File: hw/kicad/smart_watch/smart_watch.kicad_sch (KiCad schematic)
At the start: 11 parts, among them U1 STM32L476RG, U2 GC9A01, U3 LIS2MDL, U4 SHT41

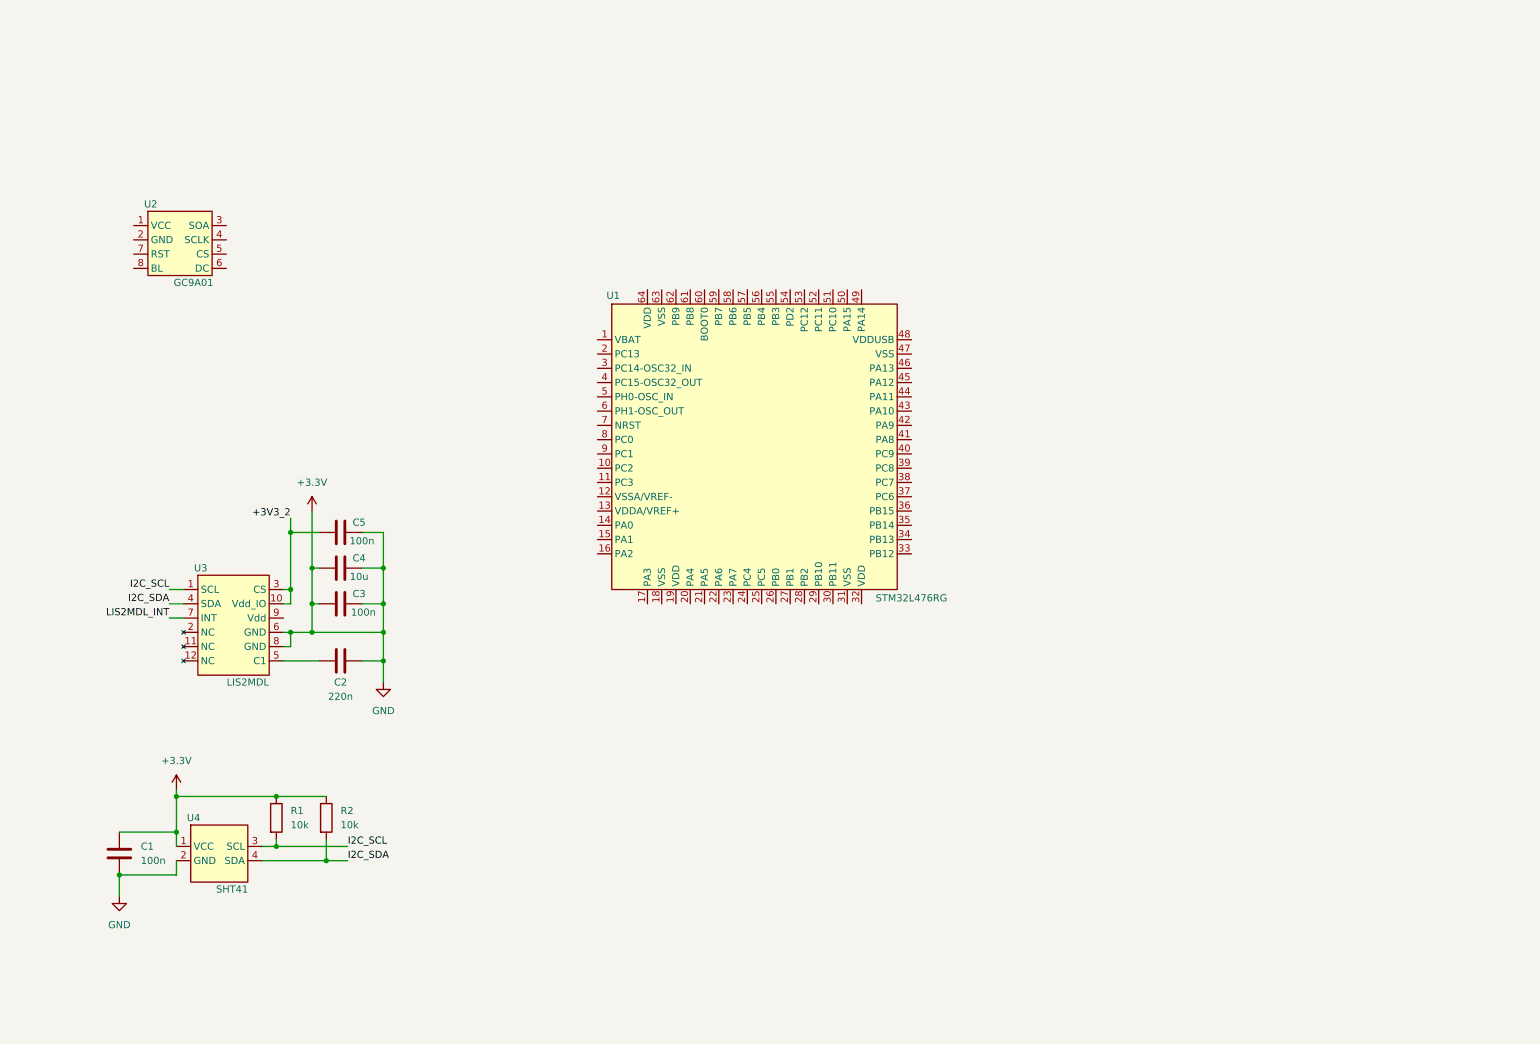
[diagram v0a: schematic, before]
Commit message: work on kicad schematic
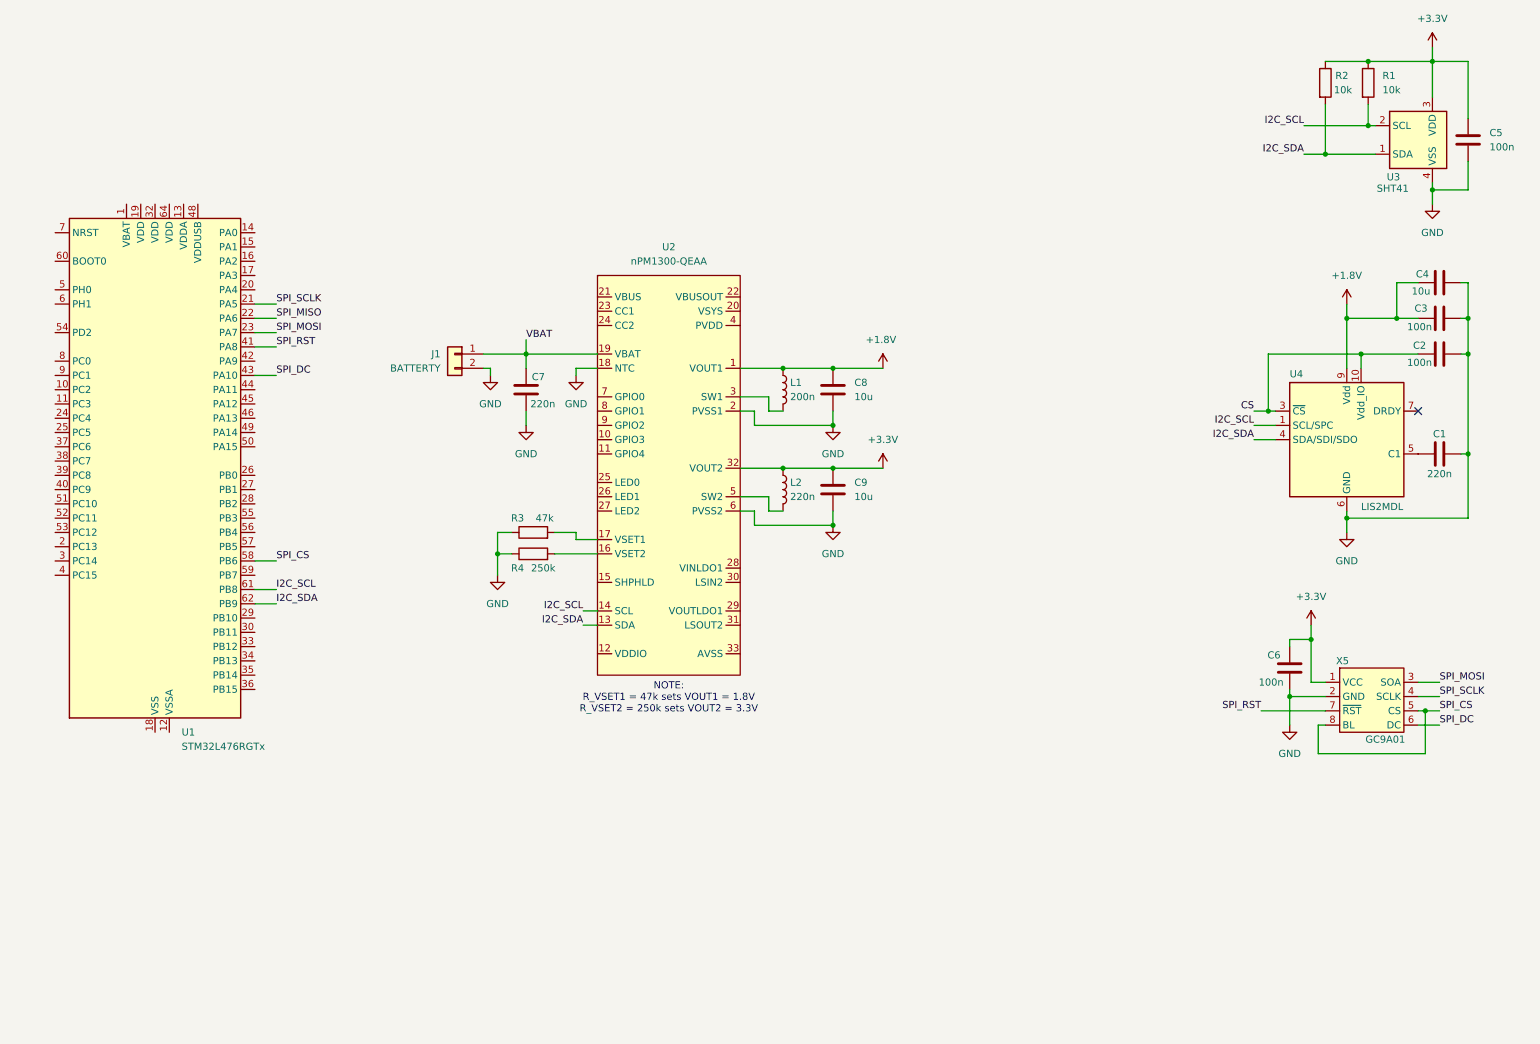
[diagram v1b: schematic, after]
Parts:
- removed U1: STM32L476RG, symbol smart_watch:STM32L476RG
- removed U2: GC9A01, symbol smart_watch:GC9A01
- removed U3: LIS2MDL, symbol smart_watch:LIS2MDL
- removed U4: SHT41, symbol smart_watch:SHT41
- added C6: 100n, symbol Device:C
- added C7: 220n, symbol Device:C
- added C8, C9: 10u, symbol Device:C
- added J1: BATTERTY, symbol Connector_Generic:Conn_01x02
- added L1: 200n, symbol Device:L
- added L2: 220n, symbol Device:L
- added R3: 47k, symbol Device:R
- added R4: 250k, symbol Device:R
- added U1: STM32L476RGTx, Package_QFP:LQFP-64_10x10mm_P0.5mm, symbol MCU_ST_STM32L4:STM32L476RGTx
- added U2: nPM1300-QEAA, symbol smart_watch:nPM1300-QEAA
- added U3: SHT41, Sensor_Humidity:Sensirion_DFN-4_1.5x1.5mm_P0.8mm_SHT4x_NoCentralPad, symbol Sensor_Humidity:SHT4x
- added U4: LIS2MDL, Package_LGA:LGA-12_2x2mm_P0.5mm, symbol Sensor_Magnetic:LIS2MDL
- added X5: GC9A01, symbol smart_watch:GC9A01
- C1: value 100n -> 220n
- C2: value 220n -> 100n
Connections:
- net +3V3_2 is gone; now on net +3.3V: C5.1
- net +3.3V: now also C6.2, C9.1, L2.1, U2.32 (VOUT2), U3.3 (VDD), X5.1 (VCC); no longer C1.1, C1.2, C2.1, C3.1, C3.2, C4.1, C4.2, C5.2
- net I2C_SCL: now also U1.61 (PB8), U2.14 (SCL), U3.2 (SCL), U4.1 (SCL/SPC)
- net I2C_SDA: now also U1.62 (PB9), U2.13 (SDA), U3.1 (SDA), U4.4 (SDA/SDI/SDO)
- net GND: now reaches C2.2
- net GND: now also C1.2, C3.2, C4.2, C5.2, C6.1, C7.2, C8.2, C9.2, J1.2 (Pin_2), R3.1, R4.1, U2.18 (NTC), U2.2 (PVSS1), U2.6 (PVSS2), U3.4 (VSS), U4.6 (GND), U4.8 (GND), X5.2 (GND)
- new net: U1.18 (VSS), U1.31 (VSS), U1.47 (VSS), U1.63 (VSS)
- new net: R4.2, U2.16 (VSET2)
- new net: R3.2, U2.17 (VSET1)
- new net: L1.2, U2.3 (SW1)
- new net: L2.2, U2.5 (SW2)
- new net: C1.1, U4.5 (C1)
- new net +1.8V: C3.1, C4.1, C8.1, L1.1, U2.1 (VOUT1), U4.9 (Vdd)
- new net CS: C2.1, U4.10 (Vdd_IO), U4.3 (~{CS})
- new net SPI_CS: U1.58 (PB6), X5.5 (CS), X5.8 (BL)
- new net SPI_DC: U1.43 (PA10), X5.6 (DC)
- new net SPI_MISO: U1.22 (PA6)
- new net SPI_MOSI: U1.23 (PA7), X5.3 (SOA)
- new net SPI_RST: U1.41 (PA8), X5.7 (~{RST})
- new net SPI_SCLK: U1.21 (PA5), X5.4 (SCLK)
- new net VBAT: C7.1, J1.1 (Pin_1), U2.19 (VBAT)
- no-connect marks 0 -> 1
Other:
- note added: "NOTE: R_VSET1 = 47k sets VOUT1 = 1.8V R_VSET2 = 250k sets VOUT2 = 3.3V"

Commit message: schematic
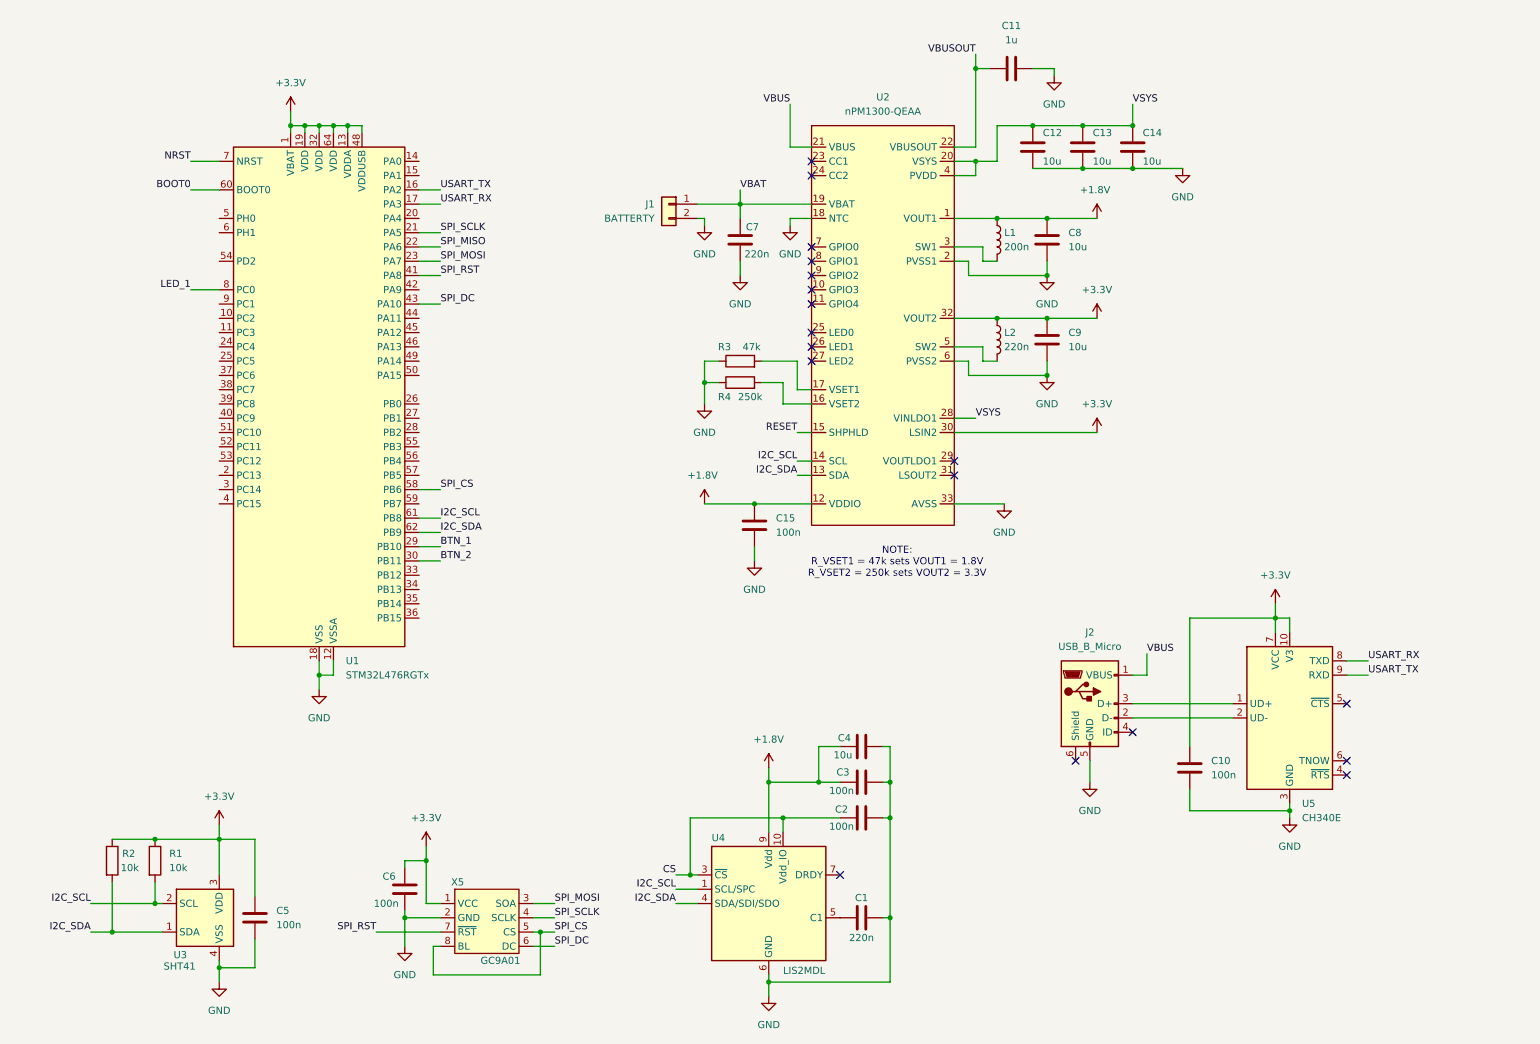
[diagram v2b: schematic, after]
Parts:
- added C10, C15: 100n, symbol Device:C
- added C11: 1u, symbol Device:C
- added C12, C13, C14: 10u, symbol Device:C
- added J2: USB_B_Micro, symbol Connector:USB_B_Micro
- added U5: CH340E, Package_SO:MSOP-10_3x3mm_P0.5mm, symbol Interface_USB:CH340E
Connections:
- net +1.8V: now also U2.12 (VDDIO), C15.1
- net +3.3V: now also U1.1 (VBAT), U1.13 (VDDA), U1.19 (VDD), U1.32 (VDD), U1.48 (VDDUSB), U1.64 (VDD), U2.30 (LSIN2), C10.1, U5.10 (V3), U5.7 (VCC)
- net GND: now also U1.12 (VSSA), U1.18 (VSS), U1.31 (VSS), U1.47 (VSS), U1.63 (VSS), U2.33 (AVSS), C10.2, C11.2, C12.1, C13.1, C14.1, C15.2, J2.5 (GND), U5.3 (GND)
- net USART_TX: now reaches U1.16 (PA2)
- net USART_TX: now also U5.9 (RXD)
- net USART_RX: now reaches U1.17 (PA3)
- net USART_RX: now also U5.8 (TXD)
- net BTN_1: now reaches U1.29 (PB10)
- net BTN_2: now reaches U1.30 (PB11)
- net BOOT0: now reaches U1.60 (BOOT0)
- net NRST: now reaches U1.7 (NRST)
- net LED_1: now reaches U1.8 (PC0)
- net RESET: now reaches U2.15 (SHPHLD)
- net VSYS: now reaches U2.20 (VSYS)
- net VSYS: now also U2.28 (VINLDO1), U2.4 (PVDD), C12.2, C13.2, C14.2
- net VBUS: now reaches U2.21 (VBUS)
- net VBUS: now also J2.1 (VBUS)
- net VBUSOUT: now reaches U2.22 (VBUSOUT)
- net VBUSOUT: now also C11.1
- new net: J2.2 (D-), U5.2 (UD-)
- new net: J2.3 (D+), U5.1 (UD+)
- no-connect marks 1 -> 18
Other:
- moved on the sheet: C1, C2, C3, C4, C5, C6, C7, C8, C9, J1, L1, L2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

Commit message: schematic done?
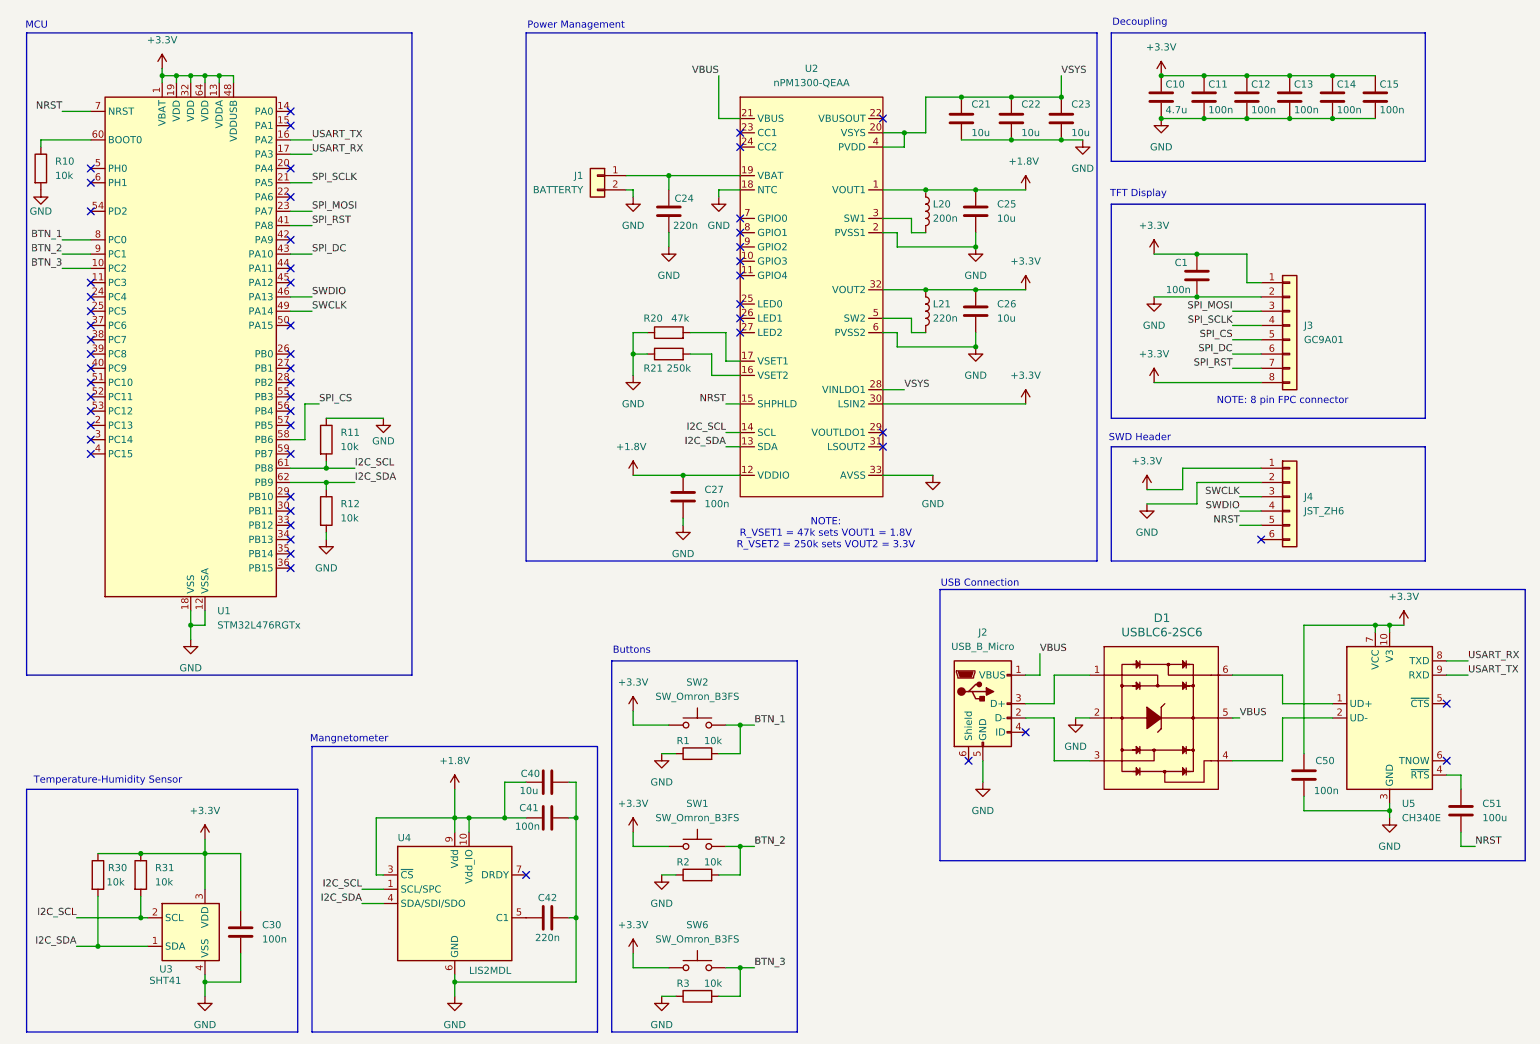
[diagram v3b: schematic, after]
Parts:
- removed C2, C6: 100n, symbol Device:C
- removed X5: GC9A01, symbol smart_watch:GC9A01
- added C1, C12, C13, C14, C15: 100n, symbol Device:C
- added C10: 4.7u, symbol Device:C
- added C51: 100u, symbol Device:C
- added D1: USBLC6-2SC6, digikey-footprints:SOT23-6L, symbol dk_TVS-Diodes:USBLC6-2SC6
- added J3: GC9A01, symbol Connector_Generic:Conn_01x08
- added J4: JST_ZH6, symbol Connector_Generic:Conn_01x06
- added R1, R10, R11, R12, R2, R3: 10k, symbol Device:R
- added SW1, SW2, SW6: SW_Omron_B3FS, symbol Switch:SW_Omron_B3FS
- C11: value 1u -> 100n
- renumbered C12 to C21, C13 to C22, C14 to C23, C7 to C24, C8 to C25, C9 to C26, C15 to C27, C5 to C30, C4 to C40, C3 to C41, C1 to C42, C10 to C50, L1 to L20, L2 to L21, R3 to R20, R4 to R21, R2 to R30, R1 to R31
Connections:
- net CS is gone; now on net +1.8V: U4.10 (Vdd_IO), U4.3 (~{CS})
- net LED_1 is gone; now on net BTN_1: U1.8 (PC0)
- net RESET is gone; now on net NRST: U2.15 (SHPHLD)
- net +3.3V: now also C11.1, C1.2, C10.1, C12.1, C13.1, C14.1, C15.1, J3.1 (Pin_1), J3.8 (Pin_8), J4.1 (Pin_1), SW1.1, SW2.1, SW6.1
- net BTN_1: now also R1.2, SW2.2; no longer U1.29 (PB10)
- net BTN_2: now also U1.9 (PC1), R2.2, SW1.2; no longer U1.30 (PB11)
- net GND: now also C1.1, C10.2, C12.2, C13.2, C14.2, C15.2, D1.2, J3.2 (Pin_2), J4.2 (Pin_2), R1.1, R10.2, R11.1, R12.2, R2.1, R3.1
- net I2C_SCL: now also R11.2
- net I2C_SDA: now also R12.1
- net NRST: now also C51.2, J4.5 (Pin_5)
- net SPI_CS: now also J3.5 (Pin_5)
- net SPI_DC: now also J3.6 (Pin_6)
- net SPI_MOSI: now also J3.3 (Pin_3)
- net SPI_RST: now also J3.7 (Pin_7)
- net SPI_SCLK: now also J3.4 (Pin_4)
- net VBUS: now also D1.5
- net BTN_3: now reaches U1.10 (PC2)
- net BTN_3: now also R3.2, SW6.2
- net SWDIO: now reaches U1.46 (PA13)
- net SWDIO: now also J4.4 (Pin_4)
- net SWCLK: now reaches U1.49 (PA14)
- net SWCLK: now also J4.3 (Pin_3)
- net at J2.2 (D-): now also D1.3; no longer U5.2 (UD-)
- net at J2.3 (D+): now also D1.1; no longer U5.1 (UD+)
- net at U5.4 (~{RTS}): now also C51.1
- net BOOT0: no longer names the net of U1.60 (BOOT0)
- net BOOT0: now also R10.1
- net SPI_MISO: no longer names the net of U1.22 (PA6)
- net VBAT: no longer names the net of C24.1, J1.1 (Pin_1), U2.19 (VBAT)
- net VBUSOUT: no longer names the net of U2.22 (VBUSOUT)
- net VBUSOUT: no longer C11.1
- new net: D1.4, U5.2 (UD-)
- new net: D1.6, U5.1 (UD+)
- no-connect marks 18 -> 56
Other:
- note added: "Buttons"
- note added: "Decoupling"
- note added: "MCU"
- note added: "Mangnetometer"
- note added: "NOTE: 8 pin FPC connector"
- note added: "Power Management"
- note added: "SWD Header"
- note added: "TFT Display"
- note added: "Temperature-Humidity Sensor"
- note added: "USB Connection"
- moved on the sheet: C21, C22, C23, C24, C25, C26, C27, C30, C40, C41, C42, C50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

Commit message: pmic footprint
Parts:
- U2: footprint (none) -> smart_watch:nPM1300
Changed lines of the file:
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@@
 			)
 		)
-		(property "Footprint" ""
+		(property "Footprint" "smart_watch:nPM1300"
 			(at 142.24 39.37 0)
 			(effects
